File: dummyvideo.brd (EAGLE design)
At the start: 34 x 27.9 mm, 14 parts, among them IC1 NE555

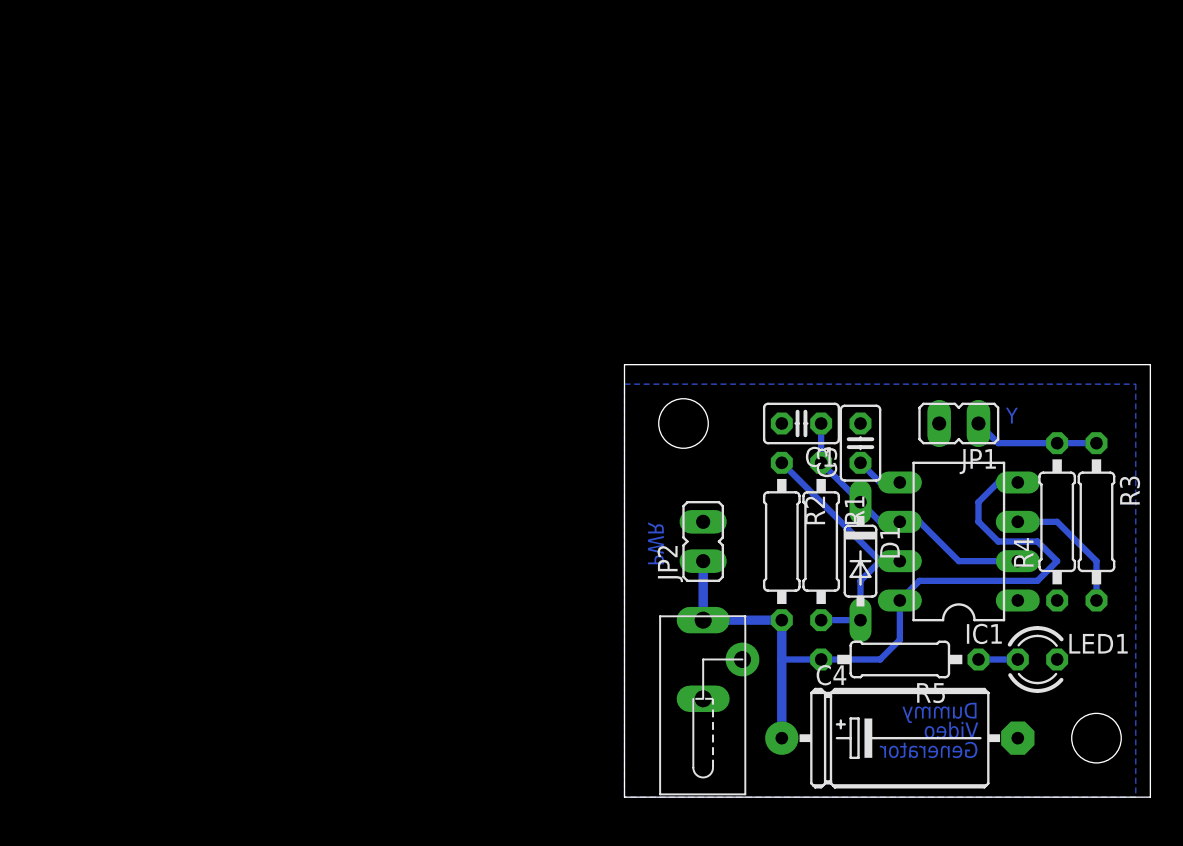
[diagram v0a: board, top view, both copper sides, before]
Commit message: First revision of SMD board
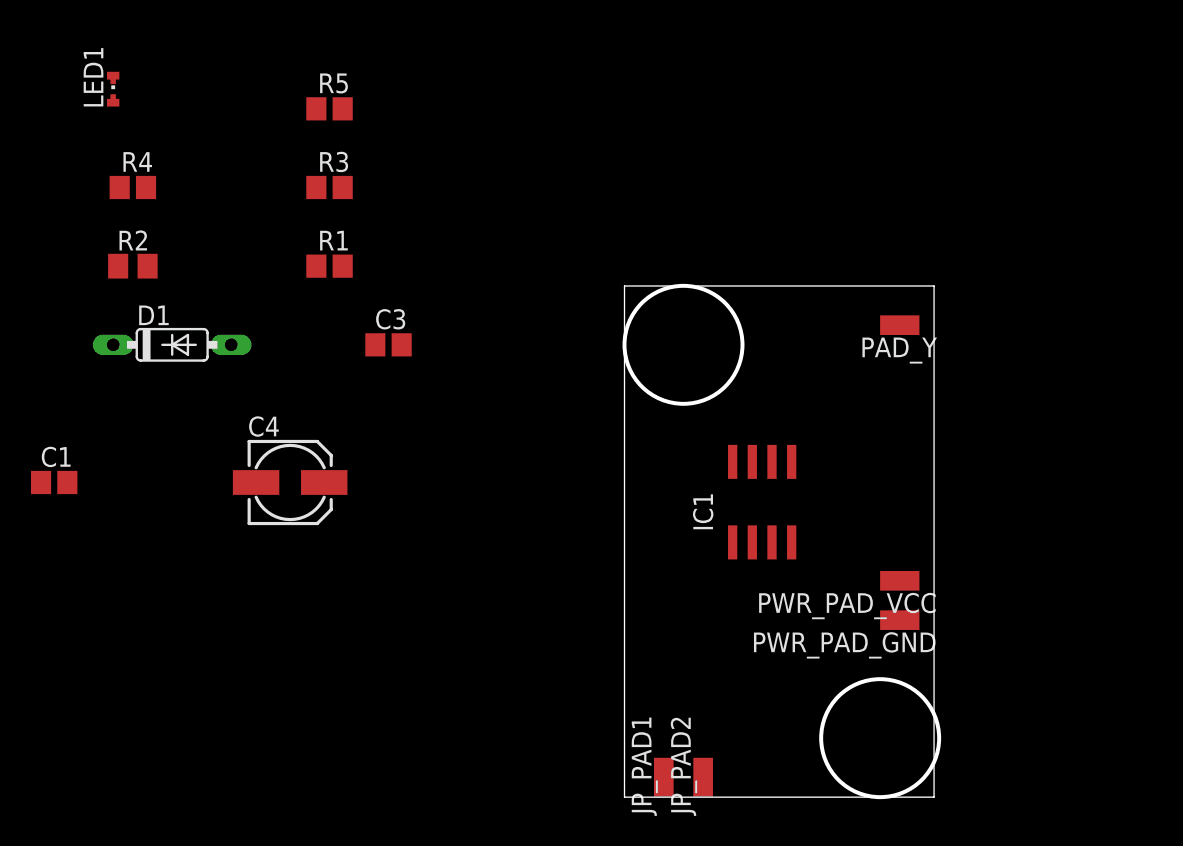
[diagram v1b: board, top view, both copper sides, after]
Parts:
- removed JP1: Y, jumper:JP1
- removed JP2: POWER, jumper:JP1
- removed U$1: DC_JACK, n39:DC_JACK_HEBO13
- added JP_PAD1, JP_PAD2, PAD_Y, PWR_PAD_GND, PWR_PAD_VCC: (no value), wirepad:SMD1,27-2,54
- C1, C3: device resistor:C025-025X050 -> resistor:C0805
- C4: value 100u -> 47u; device resistor:E15-6 -> resistor:153CLV-0505
- IC1: value NE555 -> NE555SO; device st-microelectronics:DIL-08 -> n39:SO08
- LED1: value bl -> gn LC; device led:LED3MM -> led:CHIPLED-0603-TTW
- R1, R3, R4: device resistor:0207/10 -> resistor:R0805
- R2: device resistor:0207/10 -> resistor:M0805
- R5: value 330R -> 1,5K; device resistor:0207/10 -> resistor:R0805
- moved LED1 70.1 mm to (-33.0, 45.7)
- moved R4 63.5 mm to (-31.8, 39.4), turned to 0 degrees
- moved R3 54.0 mm to (-19.1, 39.4), turned to 0 degrees
- moved R5 51.2 mm to (-19.1, 44.5), turned to 0 degrees
- moved C1 48.4 mm to (-36.8, 20.3), turned to 0 degrees
- moved D1 46.6 mm to (-29.2, 29.2), turned to 0 degrees
- moved R2 45.5 mm to (-31.8, 34.3), turned to 0 degrees
- moved C4 42.7 mm to (-21.6, 20.3)
- moved R1 36.4 mm to (-19.1, 34.3), turned to 0 degrees
- moved C3 31.1 mm to (-15.2, 29.2), turned to 0 degrees
- moved IC1 13.0 mm to (8.89, 19.1), turned to 0 degrees
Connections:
- new net N$6: JP_PAD2.1, PWR_PAD_VCC.1
- net GND: now also LED1.C@1, PWR_PAD_GND.1; no longer JP1.2, JP2.2, LED1.K, U$1.OUTER
- net N$5: now also LED1.A@1; no longer LED1.A
- net OUT: now also PAD_Y.1; no longer JP1.1
- net VCC: now also JP_PAD1.1; no longer JP2.1, U$1.INNER
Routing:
- net VCC: track 48.9 -> 0.00 mm
- net N$3: track 17.9 -> 0.00 mm
- net N$1: track 17.1 -> 0.00 mm
- net N$4: track 8.67 -> 0.00 mm
- net OUT: track 8.15 -> 0.00 mm
- net N$2: track 3.07 -> 0.00 mm
- net N$5: track 2.54 -> 0.00 mm
- removed copper zone on layer 16, net GND
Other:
- board size 34 x 27.9 mm -> 20.3 x 33 mm
- board text removed: "Dummy"
- board text removed: "Generator"
- board text removed: "PWR"
- board text removed: "Video"
- board text removed: "Y"
